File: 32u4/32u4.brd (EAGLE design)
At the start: 36.6 x 29.8 mm, 41 parts, among them J1 AVR_SPI_PRG_62X3_LOCK, Q1 16Mhz, Q2 DMMT5401, Q3 DMG2305UX

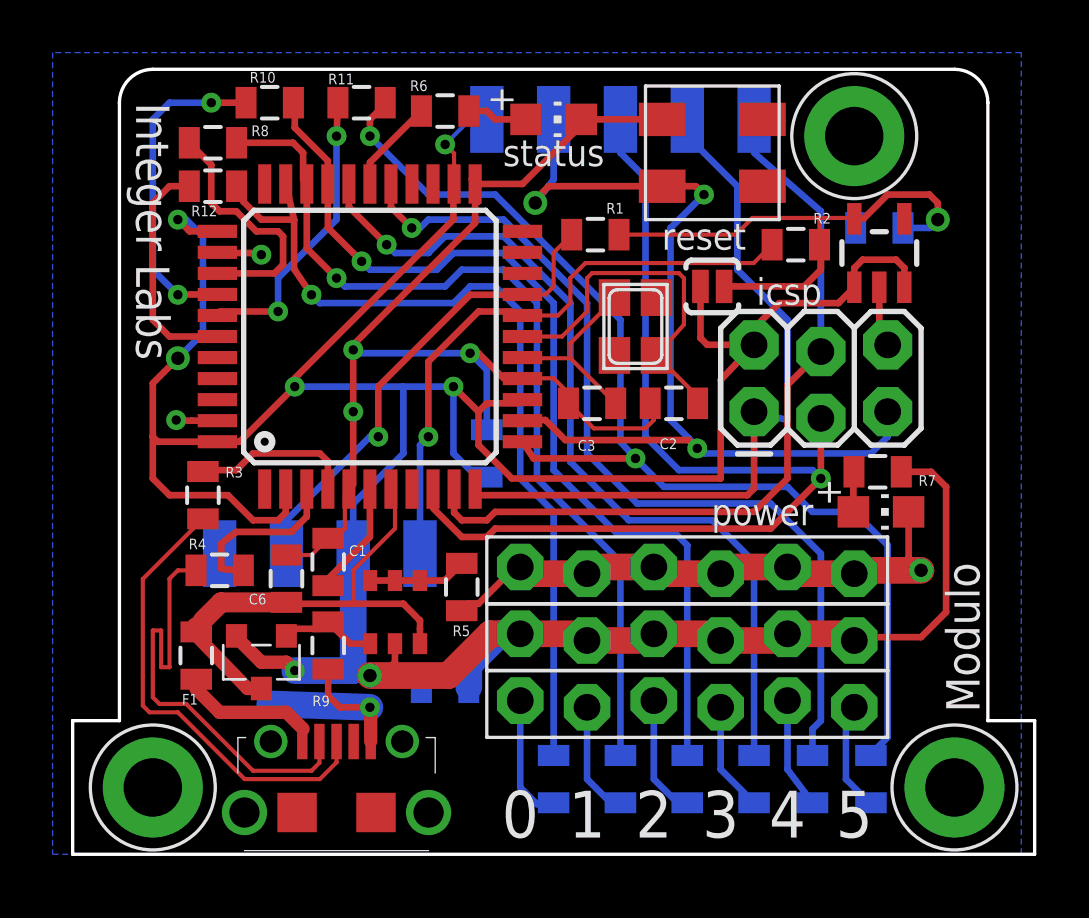
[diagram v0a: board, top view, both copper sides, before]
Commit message: Checkpointing PCB designs
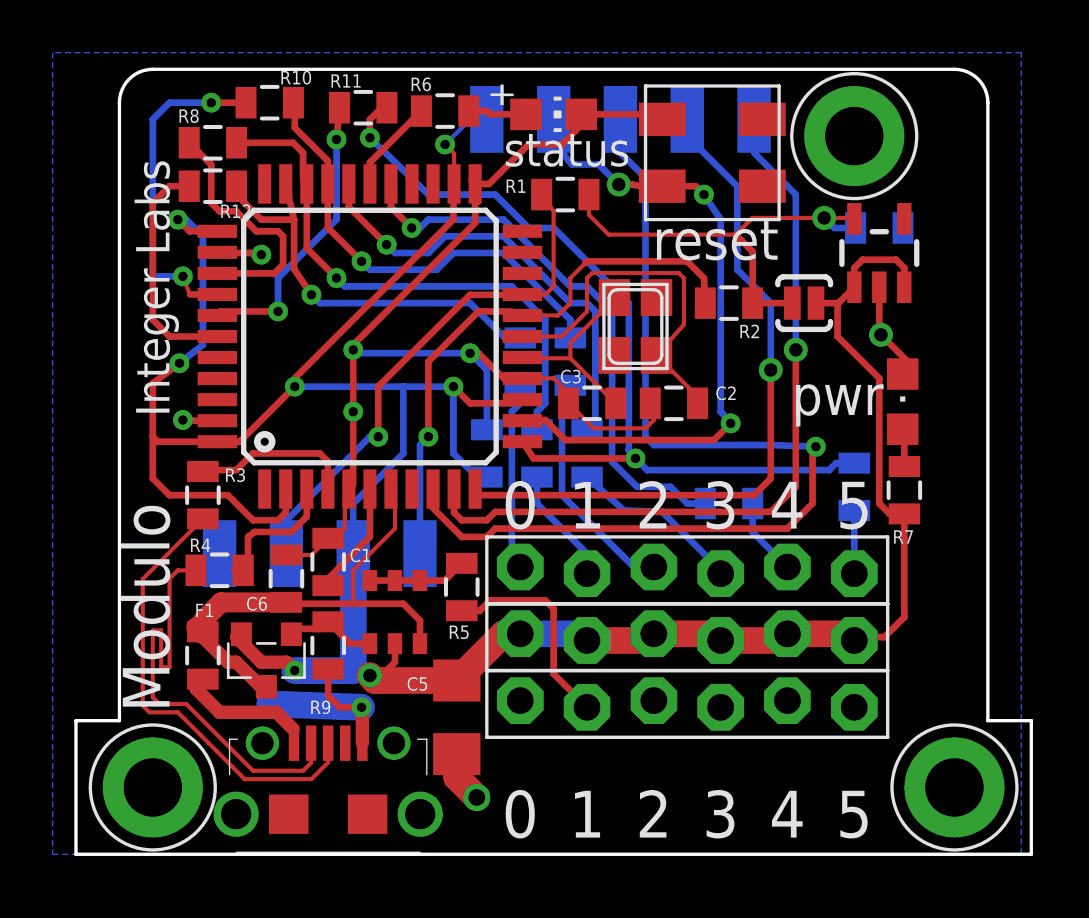
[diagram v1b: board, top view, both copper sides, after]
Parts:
- removed J1: AVR_SPI_PRG_62X3_LOCK, SparkFun-Connectors:2X3_LOCK
- C5: device SparkFun-Capacitors:0805 -> SparkFun-Capacitors:1206
- C6: value .47uF -> 10uF
- LED2: device adafruit:CHIP-LED0805 -> led:CHIPLED_0805
- R13, R14, R15, R16, R17, R18: value 220 -> 130
- moved R16 16.5 mm to (18.4, 18.7)
- moved R18 15.9 mm to (16.5, 18.7)
- moved R15 13.9 mm to (19.1, 15.2)
- moved R17 12.8 mm to (17.1, 15.2)
- moved R13 11.1 mm to (29.2, 14.0)
- moved R14 10.9 mm to (24.4, 13.3), turned to 180 degrees
- moved JP1 5.08 mm to (22.9, 10.8)
- moved JP2 5.08 mm to (22.9, 5.71)
- moved LED2 4.27 mm to (31.1, 17.2), turned to 0 degrees
- moved SJ1 3.55 mm to (27.3, 21.0), turned to 180 degrees
- moved R2 3.38 mm to (24.4, 21.0)
- moved R1 1.91 mm to (18.2, 25.1)
- moved R7 1.23 mm to (31.1, 13.8), turned to 90 degrees
- moved C5 1.23 mm to (14.1, 5.21), flipped to the top, turned to 270 degrees
- moved U$4 0.32 mm to (9.21, 1.52)
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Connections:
- net D10 renamed D2
- net D13 renamed D0
- net D6 renamed D4
- net D9 renamed D3
- removed net D11: R11.2, R13.1, U$2.12
- new net D1: R17.1, R8.2, U$2.31
- net D5: now also R11.2, R13.1, U$2.12; no longer R17.1, R8.2, U$2.31
- net GND: no longer J1.6
- net MISO: no longer J1.1
- net MOSI: no longer J1.4
- net RESET: no longer J1.5
- net SCK: no longer J1.3
- net VCC: no longer J1.2
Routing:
- net D11: track 43.3 -> 0.00 mm, vias 2 -> 0
- net VCC: track 136.6 -> 114.2 mm
- net D1: track 0.00 -> 20.9 mm, vias 0 -> 1
- net D2: track 36.2 -> 17.2 mm
- net D0: track 33.4 -> 15.9 mm
- net D3: track 33.3 -> 17.0 mm
- net D4: track 34.1 -> 21.1 mm
- net RESET: track 36.5 -> 25.0 mm
- net GND: track 80.4 -> 70.0 mm, vias 7 -> 8
- net N$18: track 4.63 -> 8.94 mm
- net +3.3V: track 20.9 -> 17.2 mm
- net N$17: track 4.16 -> 6.62 mm
- net N$20: track 4.86 -> 7.17 mm
- net D5: track 35.0 -> 33.2 mm, vias 1 -> 2
- net N$2: track 4.19 -> 2.40 mm
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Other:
- board size 36.6 x 29.8 mm -> 36.3 x 29.8 mm
- board text added: "pwr"
- board text removed: "icsp"
- board text removed: "power"
